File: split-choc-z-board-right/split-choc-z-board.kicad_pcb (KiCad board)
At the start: 2 copper layers, 122.3 x 98.6 mm, 45 parts, among them J1 USB4105-GF-A, SW1 SW_SPST, SW10 SW_SPST, SW11 SW_SPST, SW12 SW_SPST, SW13 SW_SPST, SW14 SW_SPST, SW15 SW_SPST, SW16 SW_SPST, SW17 SW_SPST, SW18 SW_SPST, SW2 SW_SPST, SW3 SW_SPST, SW4 SW_SPST, SW5 SW_SPST, SW6 SW_SPST, SW7 SW_SPST, SW8 SW_SPST, SW9 SW_SPST, U1 USBLC6-2SC6

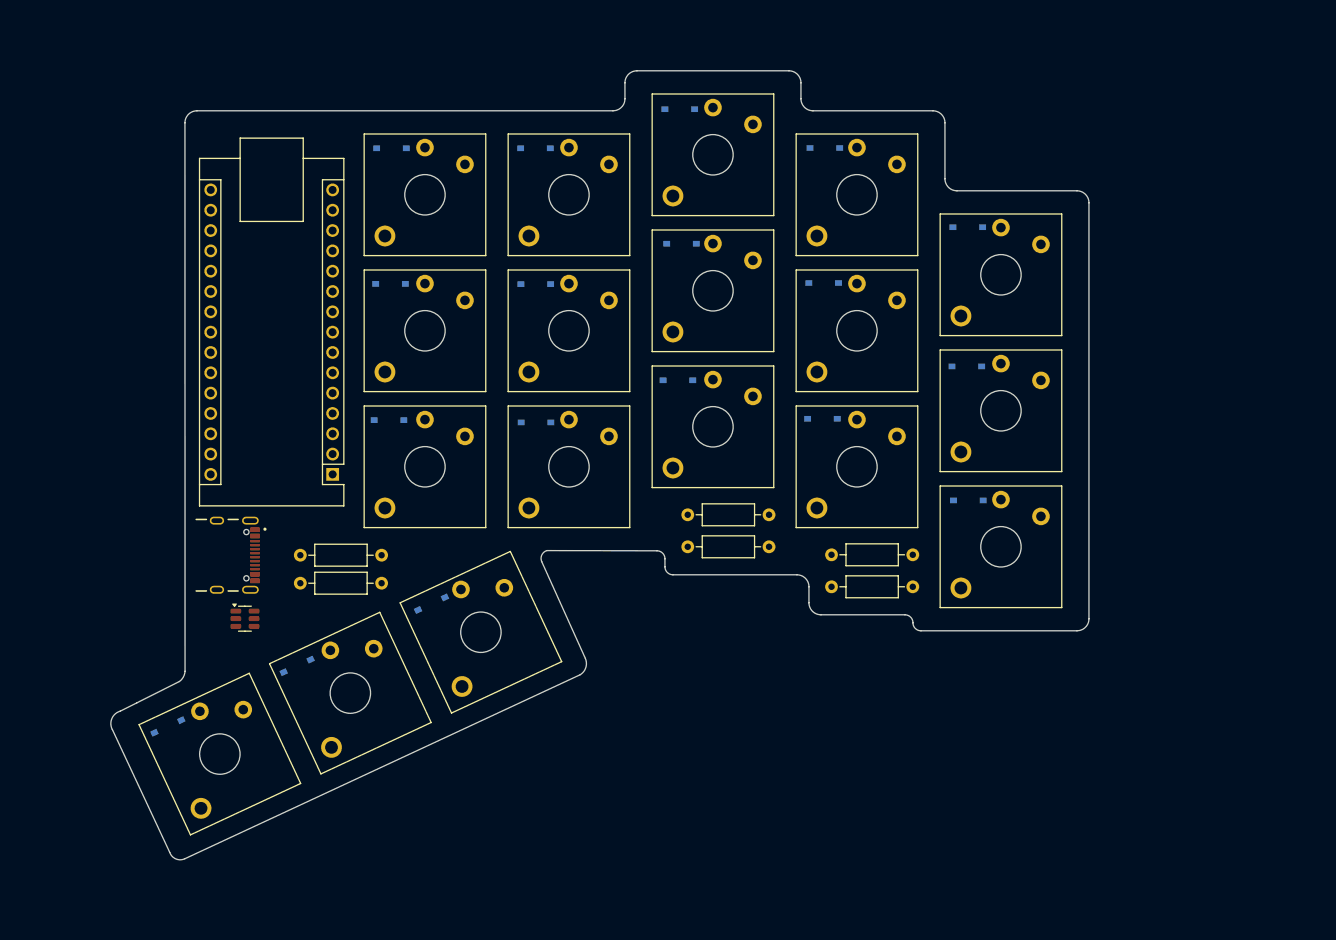
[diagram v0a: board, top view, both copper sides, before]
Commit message: Finished routing right side! 🤖
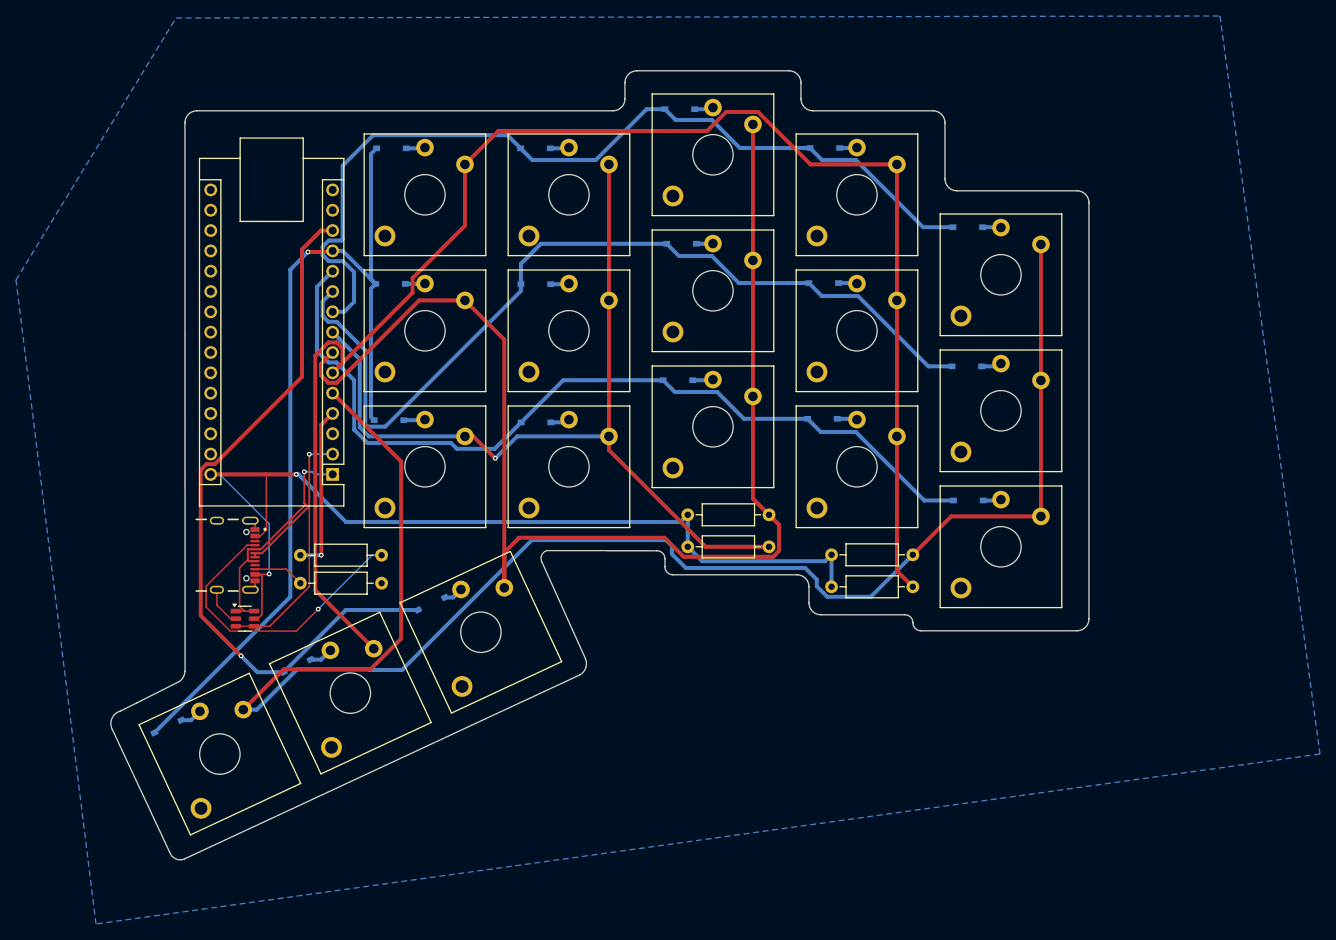
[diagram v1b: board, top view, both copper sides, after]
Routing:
- net /Column 1: track 0.00 -> 208.4 mm
- net /Column 2: track 0.00 -> 193.6 mm
- net /Column 3: track 0.00 -> 159.6 mm
- net +5V: track 0.00 -> 123.1 mm, vias 0 -> 2
- net /Row 4: track 0.00 -> 113.2 mm, vias 0 -> 1
- net /Row 1: track 0.00 -> 112.7 mm
- net /Row 2: track 0.00 -> 111.2 mm
- net /Row 3: track 0.00 -> 108.8 mm
- net /Column 4: track 0.00 -> 107.9 mm, vias 0 -> 1
- net /Row 5: track 0.00 -> 89.7 mm, vias 0 -> 1
- net /RX: track 0.00 -> 40.4 mm, vias 0 -> 1
- net /CC1: track 0.00 -> 37.9 mm, vias 0 -> 1
- net /TX: track 0.00 -> 29.1 mm, vias 0 -> 1
- net GND: track 0.00 -> 28.6 mm, vias 0 -> 1
- net /CC2: track 0.00 -> 6.39 mm
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- added copper zone on B.Cu, net GND
